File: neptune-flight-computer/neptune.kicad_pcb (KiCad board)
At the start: 4 copper layers, 39 x 60 mm, 65 parts, among them J1 THD2528-11SD-GF, J2 Conn_01x02, J3 Conn_Coaxial, J4 USB_B_Micro, J5 Conn_01x04, J6 Conn_01x04, J7 Conn_01x04, Q1 Si2301-TP, Q2 AO3401A, SW1 TS-1187A-B-A-B, SW2 TS-1187A-B-A-B, U1 ADR5040ARTZ-2.048, U2 LM393, U3 TPS54331D, U4 AP2210N-3.3TRG1, U5 RFM95W-915S2, U6 USBLC6-2SC6, U7 STM32F411RETx, U8 BMX055, Y1 32.768k, Y2 12MHz

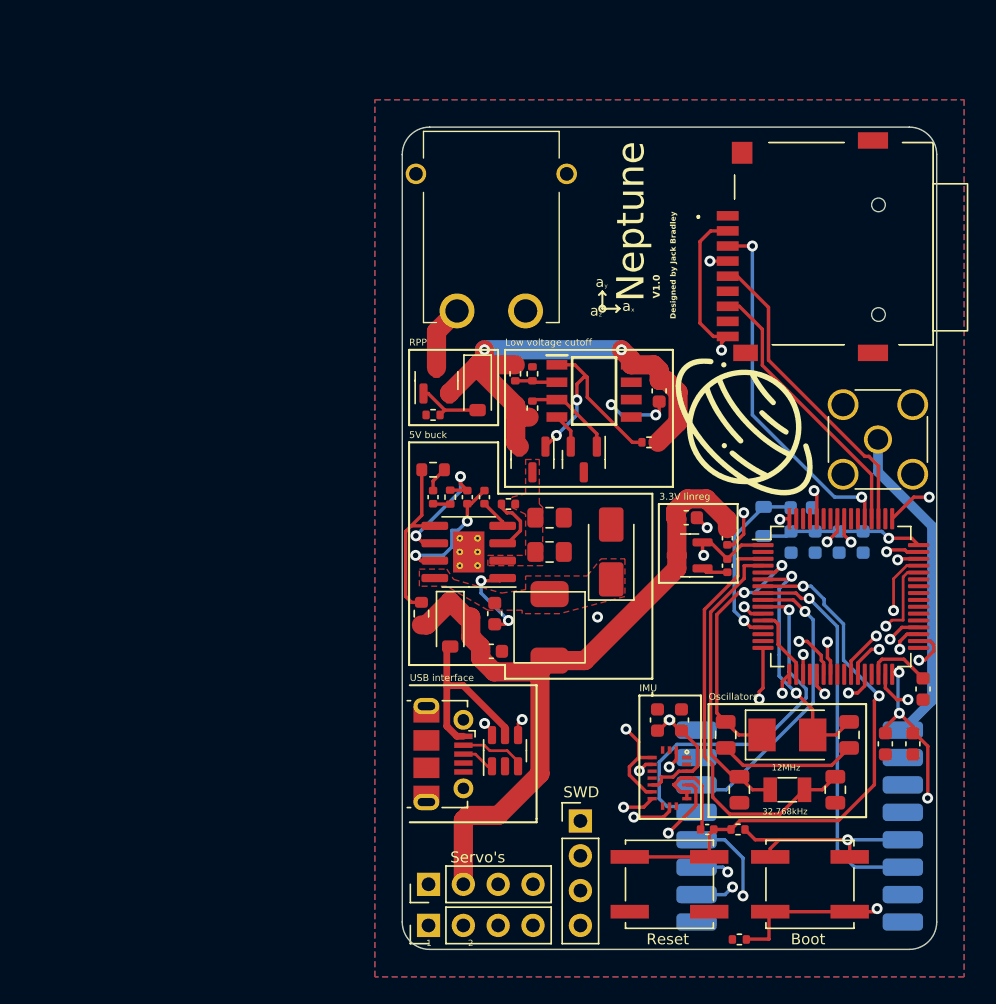
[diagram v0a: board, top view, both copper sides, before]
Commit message: Changes
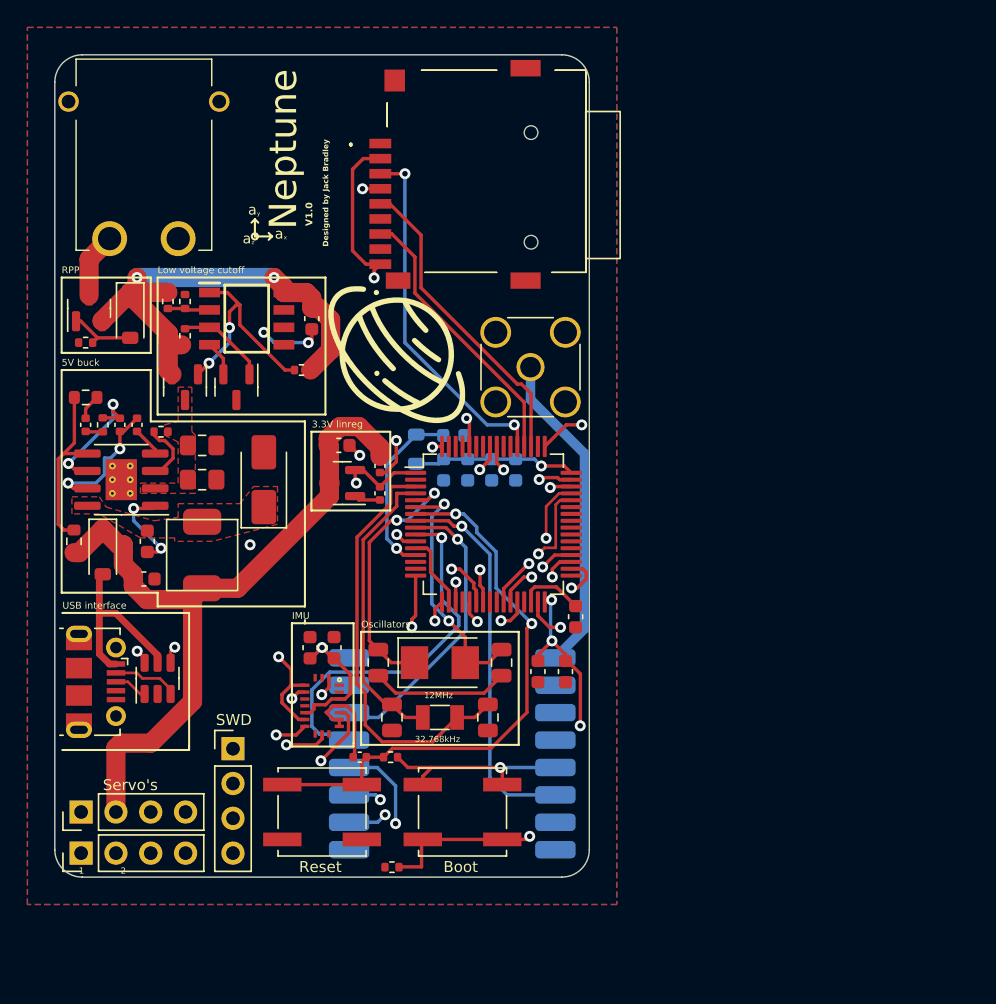
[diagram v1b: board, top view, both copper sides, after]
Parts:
- moved C1 25.9 mm to (130.2, 112.8)
- moved C3 25.9 mm to (131.2, 108.8)
- moved C10 25.9 mm to (128.7, 94.8)
- moved C22 25.9 mm to (130.5, 94.8)
- moved C23 25.9 mm to (132.2, 94.8)
- moved C13 25.9 mm to (122.3, 94.5)
- moved C16 25.9 mm to (122.3, 96.5)
- moved C17 25.9 mm to (100.8, 91.5)
- moved C2 25.9 mm to (123.2, 112.8)
- moved C21 25.9 mm to (122.2, 108.8)
- moved C6 25.9 mm to (119.3, 93.0)
- moved D3 25.9 mm to (102.1, 100.8)
- moved G*** 25.9 mm to (123.5, 86.4)
- moved J4 25.9 mm to (101.6, 110.2)
- moved J6 25.9 mm to (100.5, 122.8)
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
